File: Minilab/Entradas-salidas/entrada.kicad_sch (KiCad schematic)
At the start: 61 parts, among them J1 Out 5V/0V, J12 Vin, J13 Conn_01x07_Pin, J14 Conn_01x07_Pin, J15 Conn_01x07_Pin, J16 Conn_01x06_Pin, J17 Vin, J18 Vin, J19 Vin, J2 Out 5V/0V, J20 Vin, J21 Vin, J22 Conn_01x06_Pin, J23 Conn_01x07_Pin, J3 Out 5V/0V, J4 Out 5V/0V, J5 Out 5V/0V, J6 Out 5V/0V, SW1 SW_SPST, SW2 SW_SPST, SW3 SW_SPST, SW4 SW_SPST, SW5 SW_SPST, SW6 SW_SPST, U1 4049, U10 NE555P

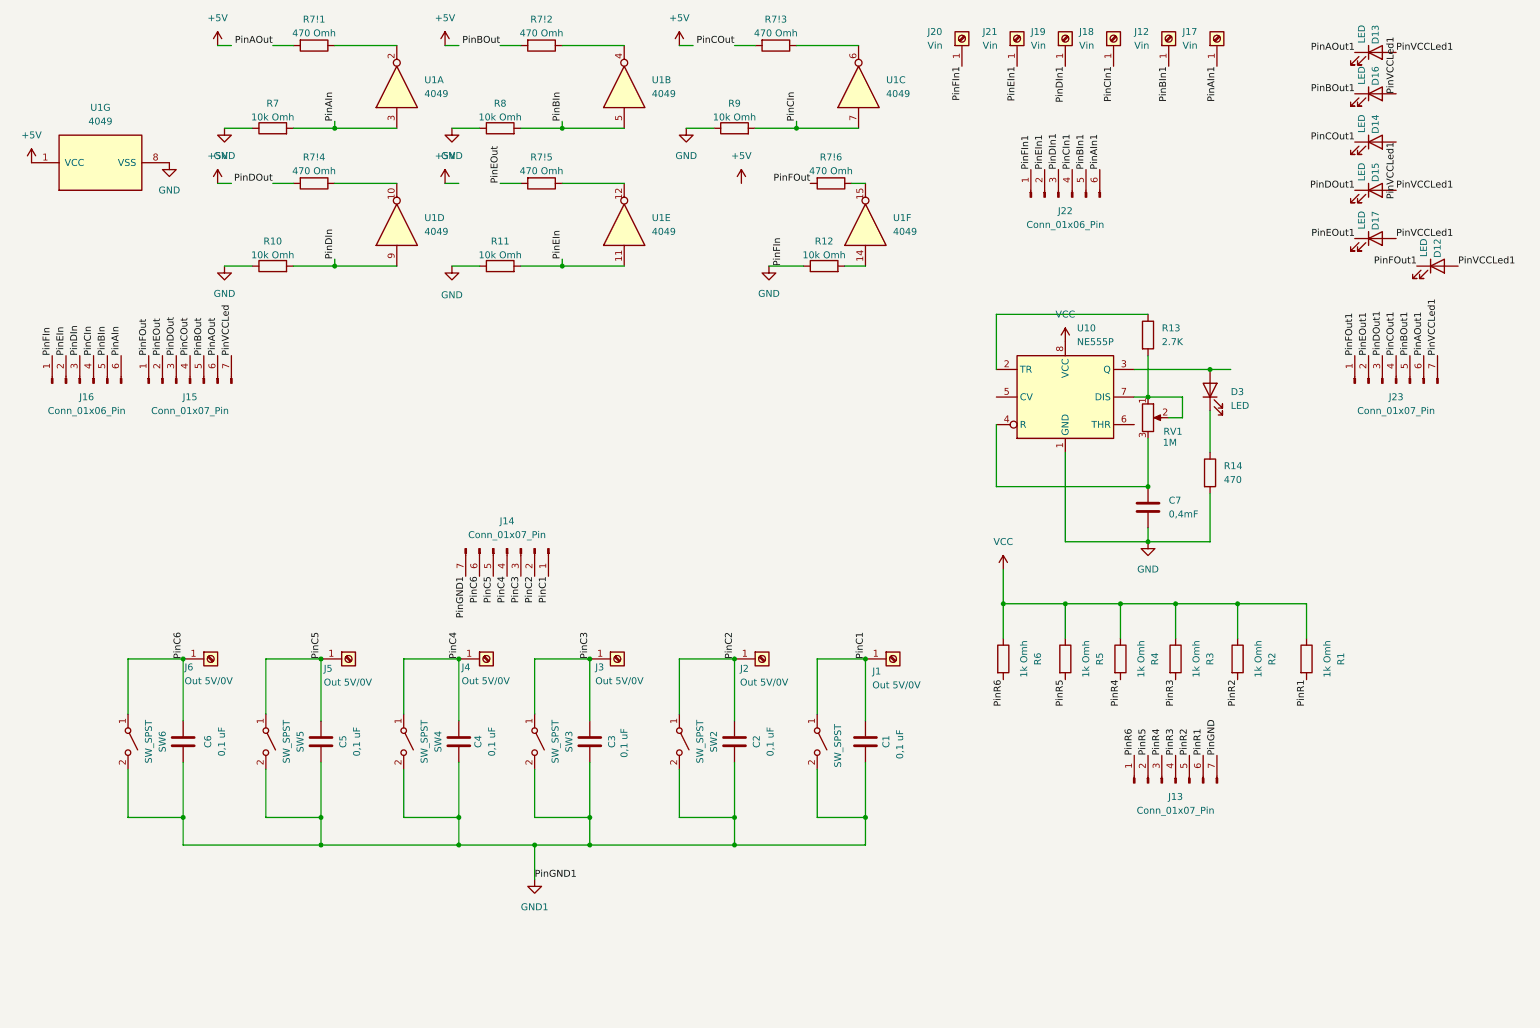
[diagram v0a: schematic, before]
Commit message: Ordeno un poco
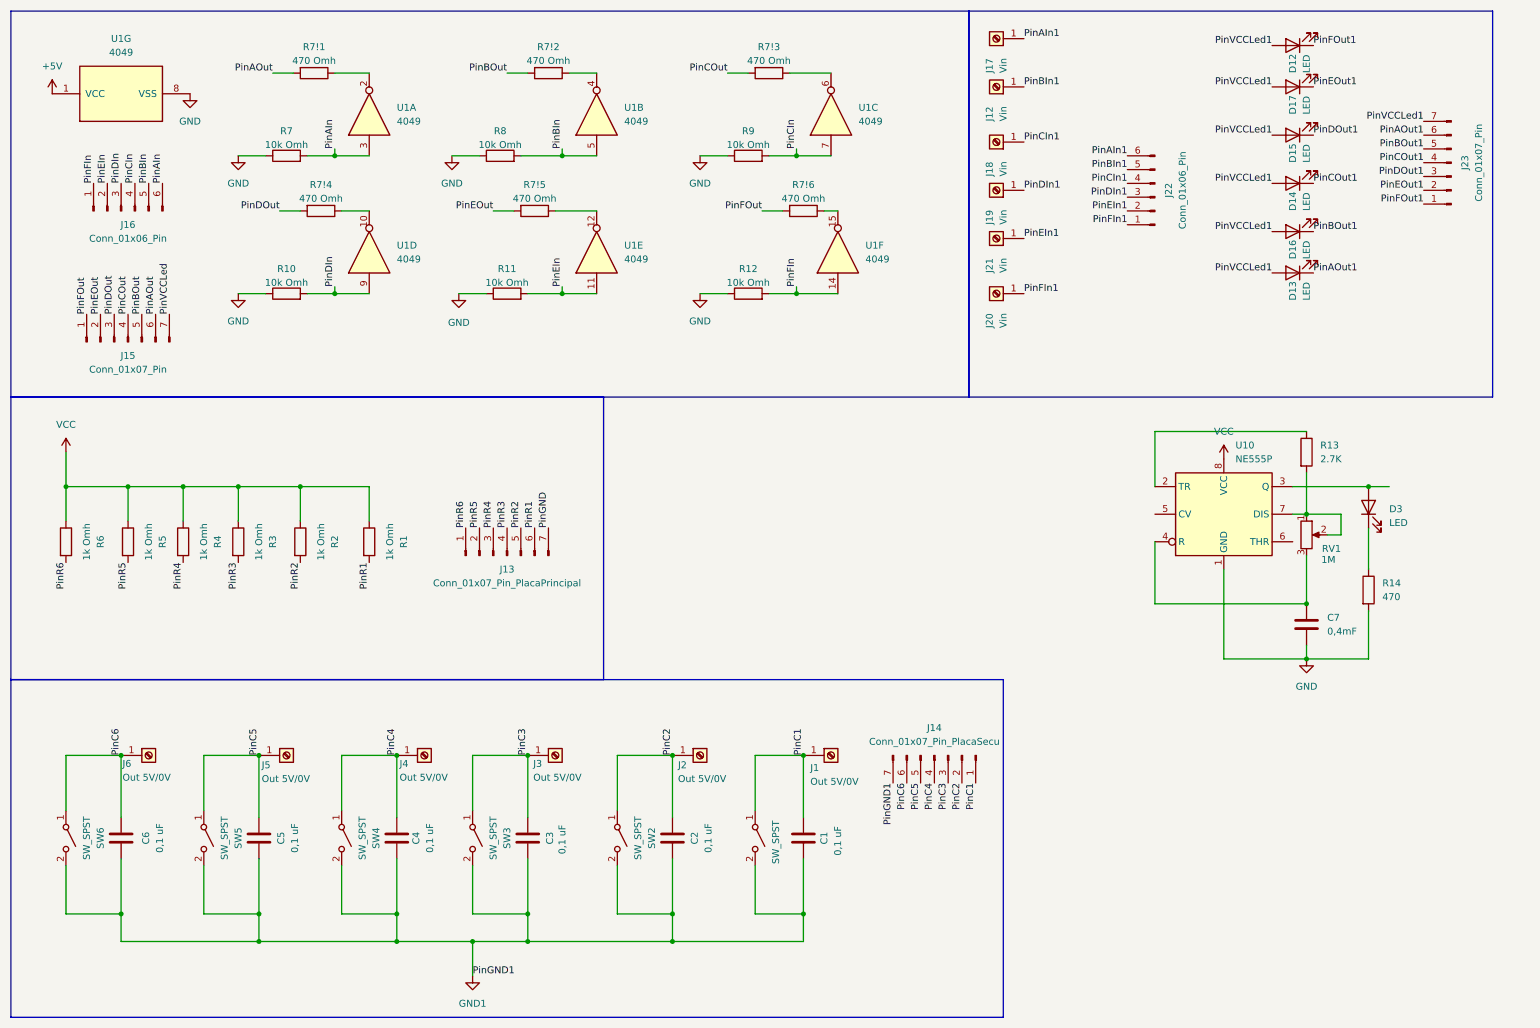
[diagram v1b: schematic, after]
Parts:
- J13: value Conn_01x07_Pin -> Conn_01x07_Pin_PlacaPrincipal
- J14: value Conn_01x07_Pin -> Conn_01x07_Pin_PlacaSecu
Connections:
- net GND: no longer J16.1 (Pin_1)
- net PinFIn: now reaches R12.2, U1.14
- net PinFIn: now also J16.1 (Pin_1)
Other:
- moved on the sheet: C1, C2, C3, C4, C5, C6, C7, D12, D13, D14, D15, D16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
